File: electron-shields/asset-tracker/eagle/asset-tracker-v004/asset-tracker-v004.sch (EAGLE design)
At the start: 30 parts, among them J1 1X2-3.5MM, T1 DMG3415, U1 MAX-M8, U2 MAX2674, U3 LIS3DHTR, U4 EPCOS-B9444, U5 MS621FE, X1 ELECTRON, X2 IPEX-20279-001E

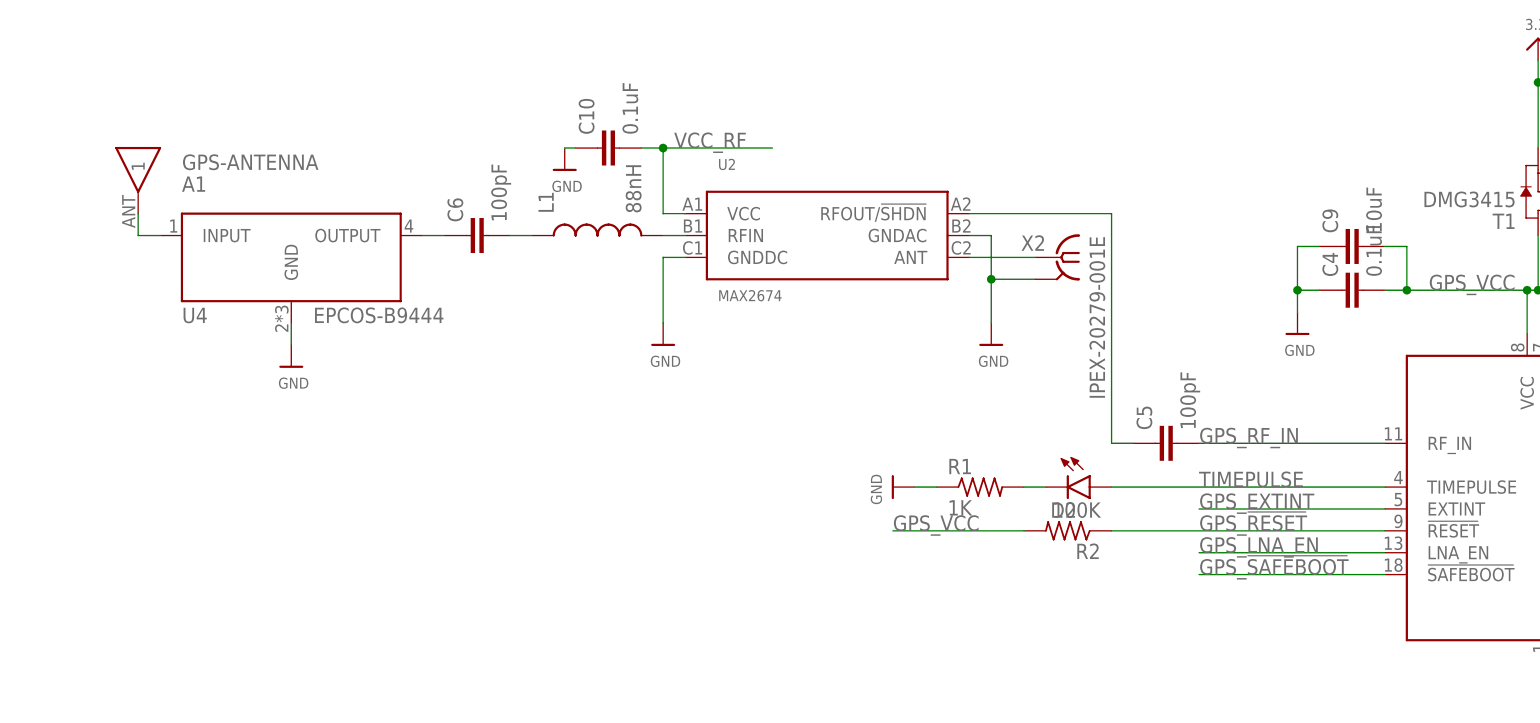
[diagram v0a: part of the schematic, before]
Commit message: added a nuclear reactor for power, routing done, need labels
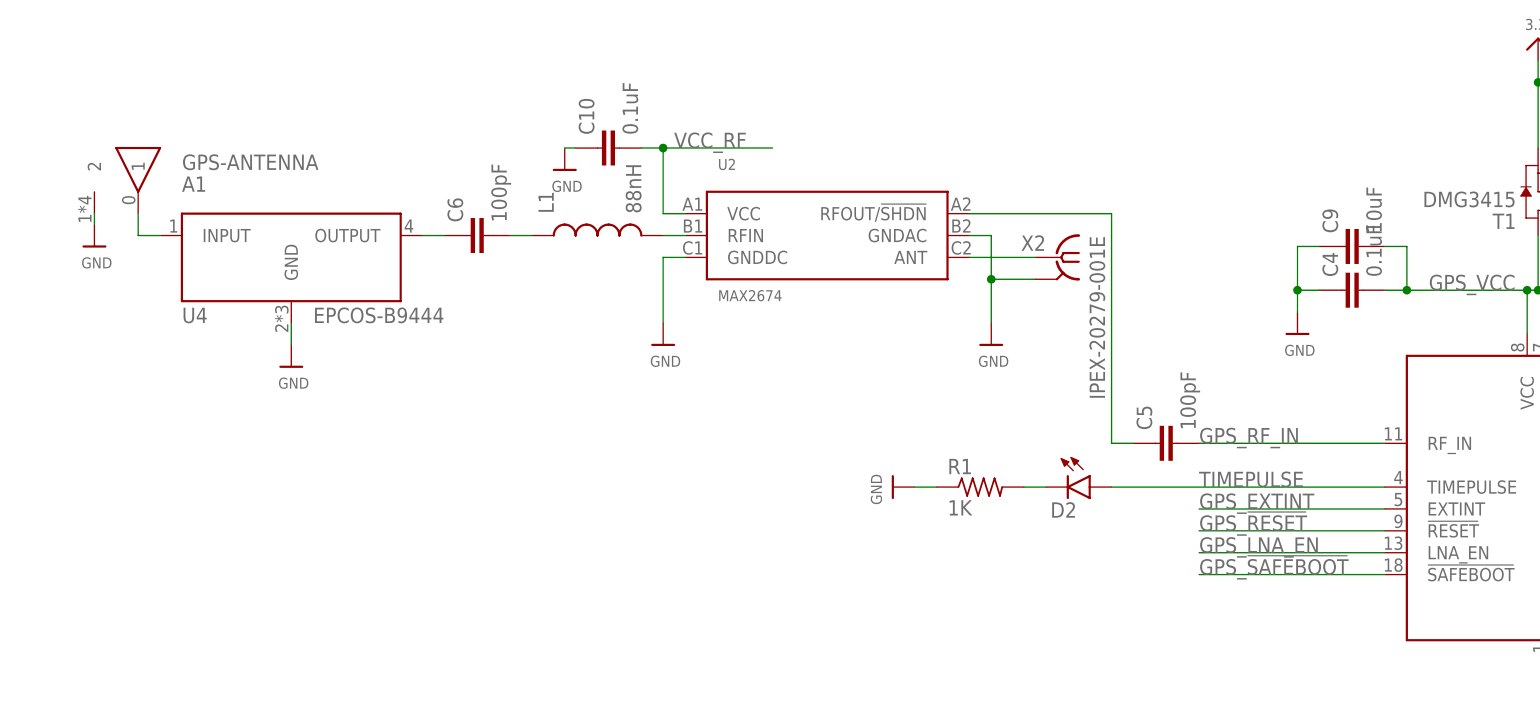
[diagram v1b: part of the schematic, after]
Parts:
- removed R2: 100K, rcl:R-US_R0402
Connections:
- net GND: now also A1.2
- net GPS_!RESET: no longer R2.1
- net GPS_VCC: no longer R2.2
